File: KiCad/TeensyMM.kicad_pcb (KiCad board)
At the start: 4 copper layers, 22 x 22 mm, 13 parts, among them J1 MICROMOD-2222, U1 MK20DX256VLH7, U2 MKL02Z32VFG4, Y2 16MHz

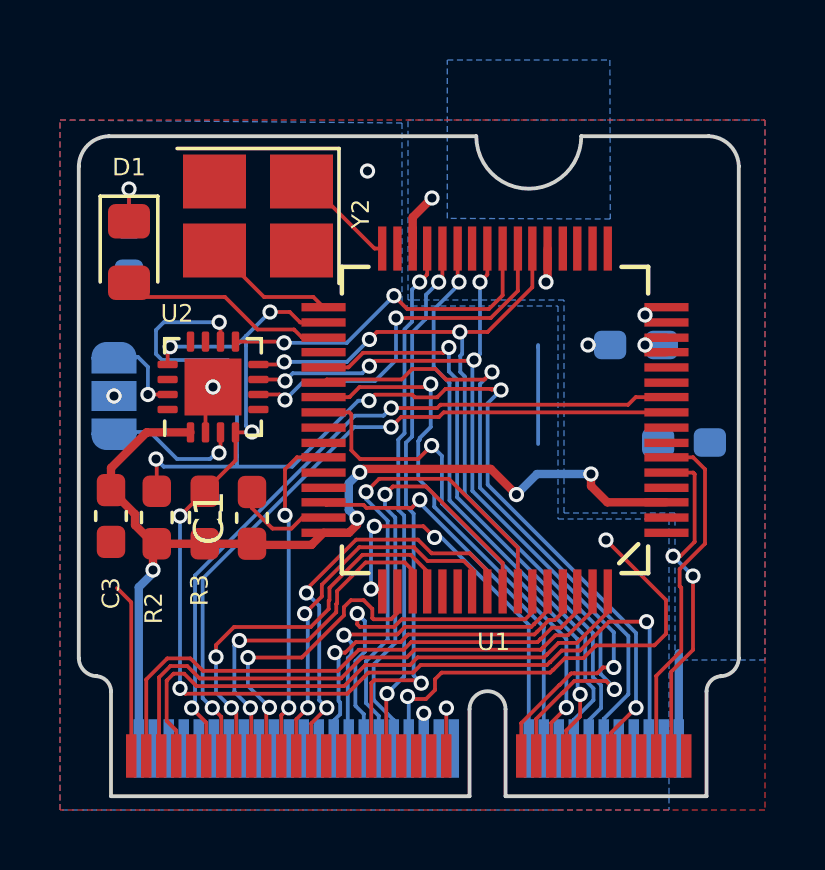
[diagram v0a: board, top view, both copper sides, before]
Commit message: wip
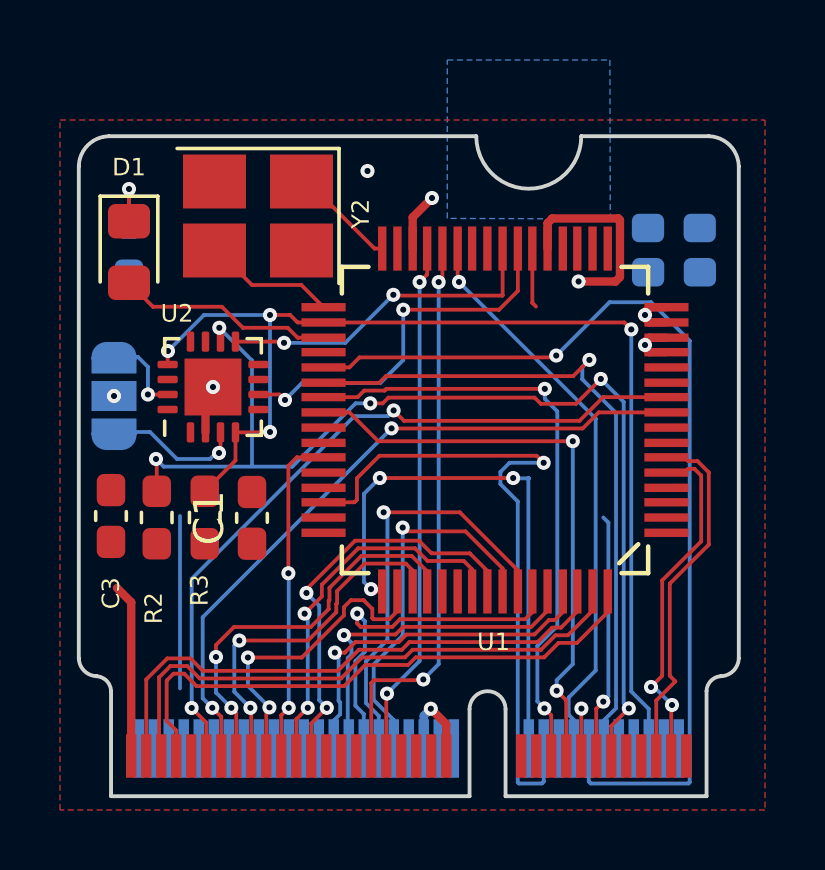
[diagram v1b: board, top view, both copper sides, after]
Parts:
- moved C2 5.68 mm to (155.0, 100.1)
- moved C4 4.10 mm to (155.0, 98.6)
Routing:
- net +3V3: track 42.0 -> 10.4 mm, vias 8 -> 3
- net SWD_DIO: track 28.6 -> 0.00 mm, vias 5 -> 0
- net SWD_CLK: track 30.1 -> 1.99 mm, vias 4 -> 0
- net /A13: track 15.5 -> 0.00 mm, vias 2 -> 0
- net /D19: track 20.1 -> 32.9 mm
- net /D9: track 13.5 -> 22.7 mm
- net /RTS: track 0.00 -> 8.19 mm, vias 0 -> 1
- net GND: track 19.4 -> 12.5 mm, vias 7 -> 5
- net /D10: track 13.4 -> 18.6 mm
- net RESET: track 41.6 -> 45.1 mm, vias 6 -> 4
- net /D14: track 17.5 -> 14.9 mm
- net /D2: track 15.7 -> 13.2 mm
- net BOOT: track 38.5 -> 36.1 mm
- net /D1: track 18.4 -> 20.2 mm
- net /D0: track 18.6 -> 20.4 mm
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- removed copper zone on B.Cu, net +3V3
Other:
- net class Default: via_dia 0.508 -> 0.4699; via_drill 0.3 -> 0.2032
- net class PWR: via_dia 0.508 -> 0.635; via_drill 0.3 -> 0.381
- rule via_min_drill: 0.3 -> 0.2032
- rule via_min_size: 0.508 -> 0.4699

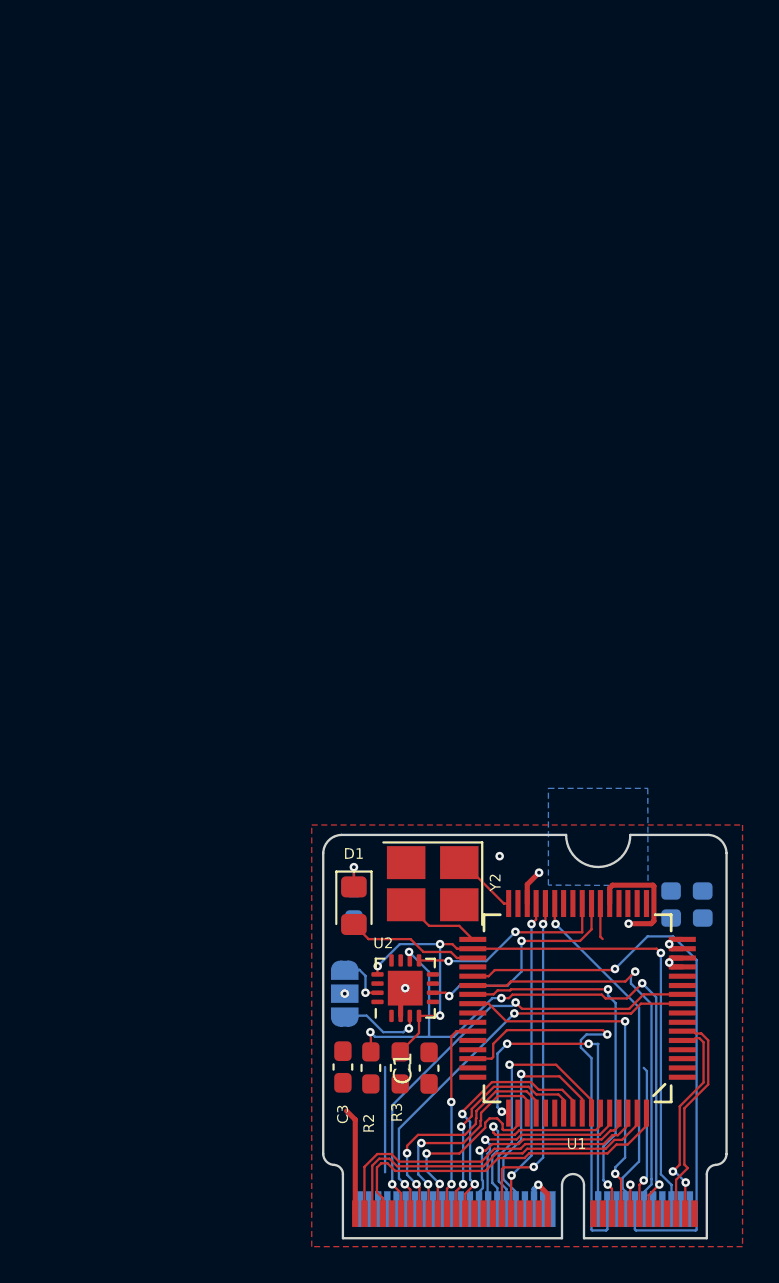
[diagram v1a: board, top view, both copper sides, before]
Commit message: finalized 4layer design
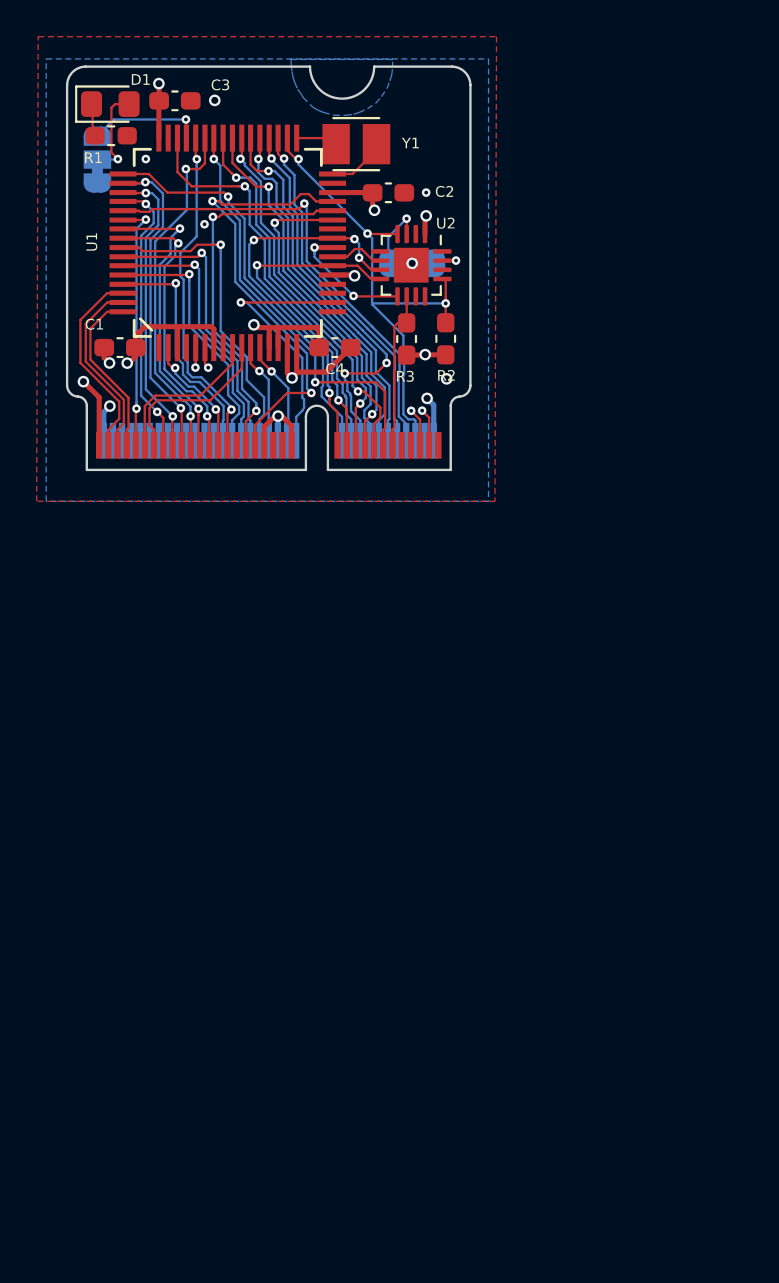
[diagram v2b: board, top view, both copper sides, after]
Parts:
- removed Y2: 16MHz, Crystal:Crystal_SMD_3225-4Pin_3.2x2.5mm_HandSoldering
- added JP2: SolderJumper_3_Bridged12, Jumper:SolderJumper-3_P1.3mm_Bridged12_RoundedPad1.0x1.5mm, B.Cu at (122.8, 58.7)
- added Y1: 16MHz, footprints:OSC_XRCHA16M000F0A01R0, F.Cu at (136.9, 57.9)
- C2, C4, R1: moved to F.Cu
- moved C3 53.5 mm to (127.0, 55.5), turned to 0 degrees
- moved U1 45.9 mm to (129.9, 63.2), turned to 90 degrees
- moved D1 45.7 mm to (123.5, 55.7), turned to 0 degrees
- moved J1 44.2 mm to (132.2, 75.6)
- moved R1 43.9 mm to (123.6, 57.4), turned to 0 degrees
- moved C2 42.8 mm to (138.7, 60.5)
- moved C1 42.8 mm to (124.0, 69.0), turned to 180 degrees
- moved JP1 40.0 mm to (140.0, 64.4), turned to 180 degrees
- moved R2 39.8 mm to (141.8, 68.5)
- moved R3 39.8 mm to (139.7, 68.5)
- moved U2 39.4 mm to (139.9, 64.5), turned to 270 degrees
- moved C4 35.3 mm to (135.8, 69.0), turned to 0 degrees
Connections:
- net /D0 renamed D00-RX1
- net /D1 renamed D01-TX1
- net /D10 renamed D10-TX2
- net /D11 renamed D11-MOSI
- net /D12 renamed D12-MISO
- net /D13 renamed D13-SCK
- net /D14 renamed D14-PTD1
- net /D15 renamed D15-CS
- net /D18 renamed D18-SDA0
- net /D19 renamed D19-SCL0
- net /D2 renamed D02-PTD0
- net /D20 renamed D20-PTD5
- net /D21 renamed D21-PTD6
- net /D24 renamed D24-I2C-INT
- net /D29 renamed D29-SCL1
- net /D30 renamed D30-SDA1
- net /D3_CTX renamed D03-CAN-TX
- net /D4_CRX renamed D04-CAN-TX
- net /D5 renamed D05-PTD7
- net /D6 renamed D06-PTD4
- net /D7 renamed D07-PTD2
- net /D8 renamed D08-PTD3
- net /D9 renamed D09-RX2
- net Net-(JP1-Pad1) renamed /PTA1
- net Net-(JP1-Pad3) renamed /PTA3
- J1 pad 10: (no net) -> D16_A2
- J1 pad 13: (no net) -> D25-RTS1
- J1 pad 15: (no net) -> D32-CTS1
- J1 pad 18: (no net) -> D17_A3
- J1 pad 32: (no net) -> DAC
- J1 pad 34: /A12 -> ADC1_N
- J1 pad 38: /A13 -> ADC1_P
- J1 pad 47: (no net) -> D22-A8
- J1 pad 49: (no net) -> D26_A15-BAT_VIN3
- J1 pad 63: /A11 -> ADC0_N
- J1 pad 65: /A10 -> ADC0_P
- J1 pad 67: (no net) -> D27_A16
- J1 pad 8: (no net) -> D28_A17
- U1 pad 10: /A10 -> ADC0_N
- U1 pad 11: /A12 -> ADC1_P
- U1 pad 12: /A13 -> ADC1_N
- U1 pad 18: (no net) -> DAC
- U1 pad 2: (no net) -> D26_A15-BAT_VIN3
- U1 pad 35: Net-(D1-Pad2) -> D16_A2
- U1 pad 36: (no net) -> D17_A3
- U1 pad 41: (no net) -> D32-CTS1
- U1 pad 42: (no net) -> D25-RTS1
- U1 pad 44: (no net) -> D22-A8
- U1 pad 45: (no net) -> D23
- U1 pad 53: (no net) -> D28_A17
- U1 pad 54: (no net) -> D27_A16
- U1 pad 9: /A11 -> ADC0_P
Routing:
- net BOOT: track 36.1 -> 8.72 mm, vias 5 -> 0
- net D28_A17: track 0.00 -> 26.1 mm, vias 0 -> 1
- net /A10: track 24.7 -> 0.00 mm, vias 2 -> 0
- net /A11: track 23.4 -> 0.00 mm, vias 2 -> 0
- net D25-RTS1: track 0.00 -> 22.6 mm, vias 0 -> 2
- net SWD_DIO: track 0.00 -> 22.2 mm, vias 0 -> 4
- net D17_A3: track 0.00 -> 21.5 mm, vias 0 -> 3
- net D32-CTS1: track 0.00 -> 21.1 mm, vias 0 -> 2
- net +3V3: track 10.4 -> 30.6 mm, vias 3 -> 10
- net D16_A2: track 0.00 -> 19.3 mm, vias 0 -> 1
- net D22-A8: track 0.00 -> 18.7 mm, vias 0 -> 2
- net SWD_CLK: track 1.99 -> 19.1 mm, vias 0 -> 2
- net RESET: track 45.1 -> 28.1 mm, vias 4 -> 3
- net DAC: track 0.00 -> 14.3 mm, vias 0 -> 1
- net D27_A16: track 0.00 -> 13.8 mm, vias 0 -> 2
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- added copper zone on B.Cu, net +3V3
- removed copper zone on B.Cu, net GND
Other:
- outline, holes or cut-outs redrawn
- board text added: "D13"
- board text added: "D23"
- board text added: "DE"
- board text added: "LED"
- board text added: "PTA3"
- board text added: "PTA6"
- board text added: "lunOptics MicroMod_32 2020-12 V1.0"
